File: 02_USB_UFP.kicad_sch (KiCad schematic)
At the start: 26 parts, among them U2 PI3USB302-Ax, U3 TUSB522Px, U4 TVS2200DRVx

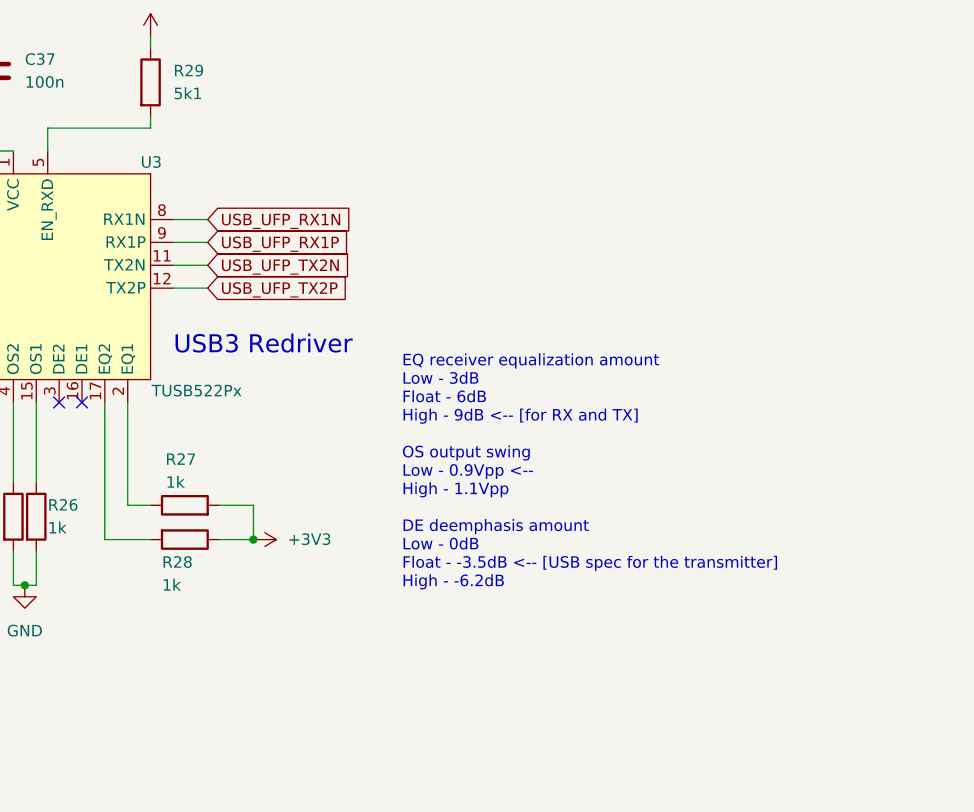
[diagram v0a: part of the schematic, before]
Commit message: WIP hub and DFP
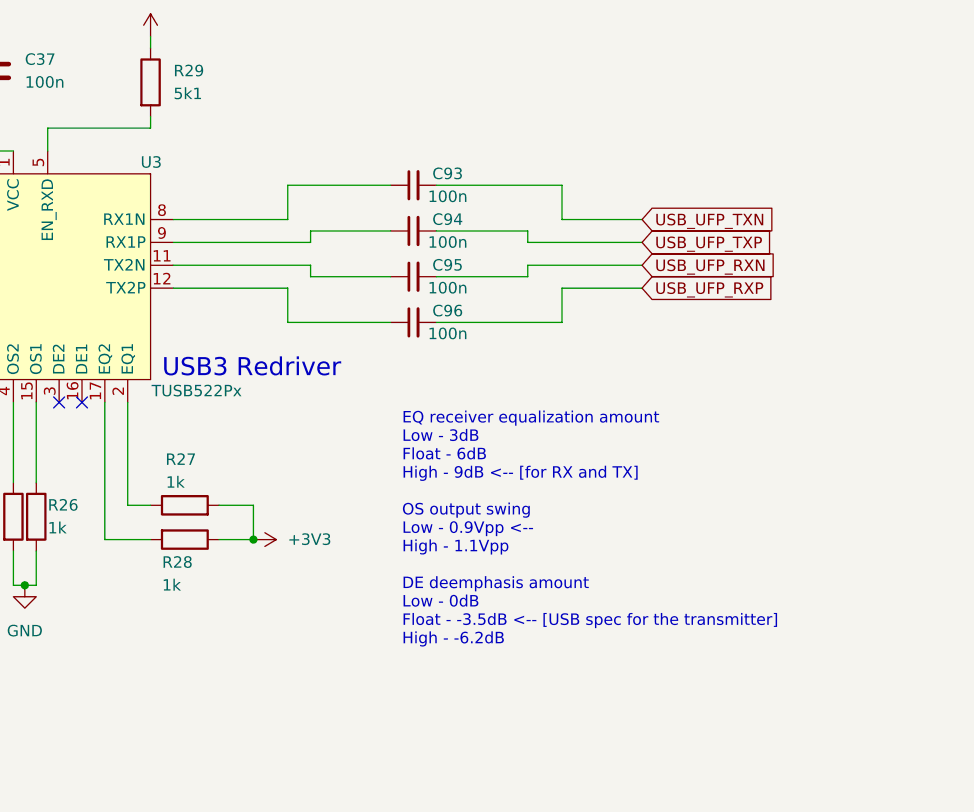
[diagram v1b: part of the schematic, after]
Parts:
- added C93, C94, C95, C96: 100n, symbol Device:C_Small
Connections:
- net USB_UFP_RX1N: no longer names the net of U3.8 (RX1N)
- net USB_UFP_RX1N: now also C93.1
- net USB_UFP_RX1P: no longer names the net of U3.9 (RX1P)
- net USB_UFP_RX1P: now also C94.1
- net USB_UFP_TX2N: no longer names the net of U3.11 (TX2N)
- net USB_UFP_TX2N: now also C95.1
- net USB_UFP_TX2P: no longer names the net of U3.12 (TX2P)
- net USB_UFP_TX2P: now also C96.1
- new net USB_UFP_RXN: C95.2
- new net USB_UFP_RXP: C96.2
- new net USB_UFP_TXN: C93.2
- new net USB_UFP_TXP: C94.2
